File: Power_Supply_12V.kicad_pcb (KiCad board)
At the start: 2 copper layers, 16 parts, among them J1 Input, J2 Output, U1 LM7812_TO220, U2 LM7912_TO220

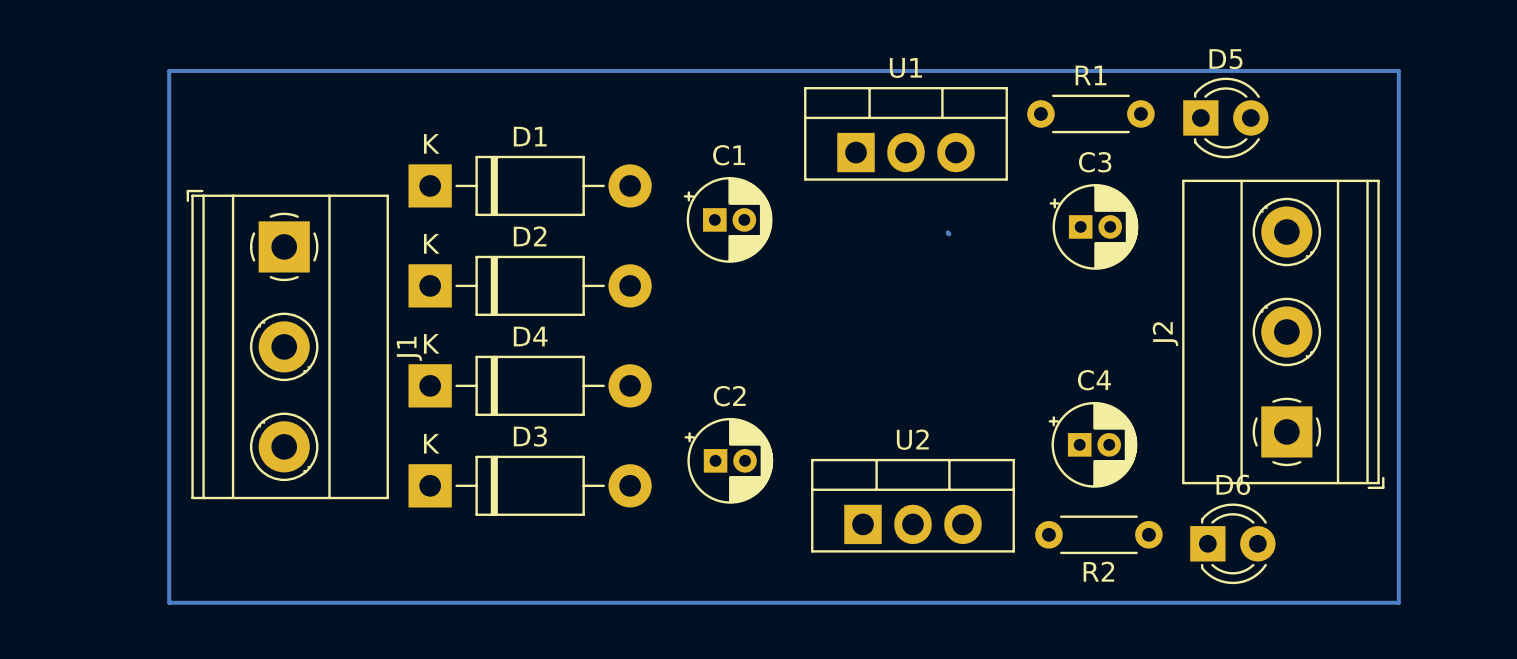
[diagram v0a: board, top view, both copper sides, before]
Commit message: Routing done
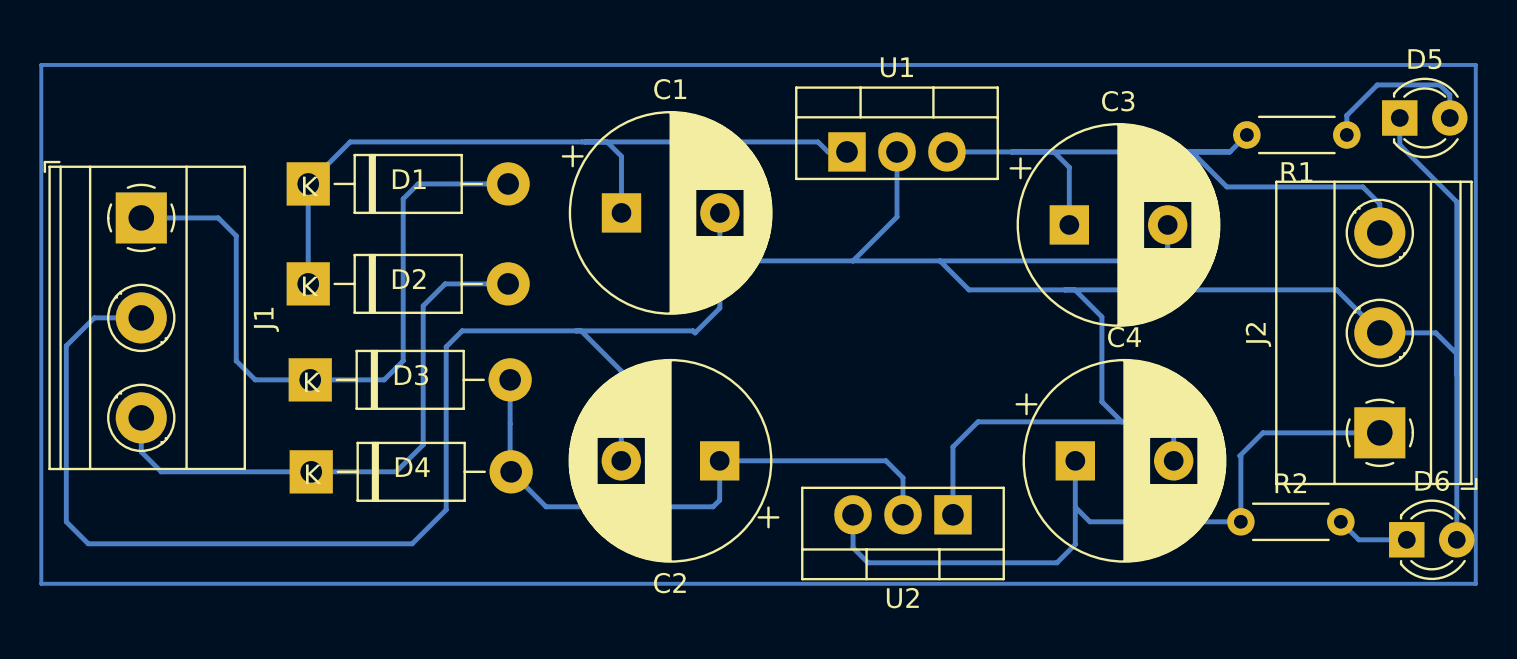
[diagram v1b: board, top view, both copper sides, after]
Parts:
- C1, C2, C3, C4: footprint Capacitor_THT:CP_Radial_D4.0mm_P1.50mm -> Capacitor_THT:CP_Radial_D10.0mm_P5.00mm
- moved R1 15.6 mm to (163.4, 68.5), turned to 180 degrees
- moved D6 10.1 mm to (166.5, 89.1)
- moved D5 10.1 mm to (166.1, 67.7)
- moved D3 8.13 mm to (110.7, 81.0)
- moved D4 7.46 mm to (110.8, 85.6)
- moved J1 7.41 mm to (102.2, 72.7)
- moved D1 6.20 mm to (110.6, 71.0)
- moved D2 6.20 mm to (110.6, 76.1)
- moved C1 4.76 mm to (126.6, 72.5)
- moved J2 4.72 mm to (165.1, 83.7)
- moved R2 4.72 mm to (158.0, 88.2), turned to 0 degrees
- moved U2 4.60 mm to (143.4, 87.8), turned to 180 degrees
- moved C4 0.84 mm to (149.6, 85.1)
- moved C3 0.59 mm to (149.3, 73.1)
- moved U1 0.46 mm to (138.0, 69.4)
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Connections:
- C3 pad 1: Net-(J2-Pin_1) -> Net-(J2-Pin_3)
- C3 pad 2: Net-(C3-Pad2) -> Net-(D5-K)
- C4 pad 1: Net-(J2-Pin_3) -> Net-(J2-Pin_1)
- C4 pad 2: Net-(C3-Pad2) -> Net-(D5-K)
- R1 pad 2: Net-(J2-Pin_1) -> Net-(J2-Pin_3)
- R2 pad 1: Net-(J2-Pin_3) -> Net-(J2-Pin_1)
- U1 pad 3: Net-(J2-Pin_1) -> Net-(J2-Pin_3)
- U2 pad 3: Net-(J2-Pin_3) -> Net-(J2-Pin_1)
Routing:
- net Net-(D5-K): track 0.61 -> 177.2 mm
- net Net-(D1-K): track 0.72 -> 38.6 mm
- net Net-(J2-Pin_1): track 0.07 -> 37.6 mm
- net Net-(J2-Pin_3): track 0.00 -> 36.9 mm
- net Net-(D1-A): track 0.00 -> 34.7 mm
- net Net-(D3-A): track 0.00 -> 30.4 mm
- net Net-(D2-A): track 0.72 -> 28.9 mm
- net Net-(D5-A): track 0.00 -> 8.24 mm
- net Net-(D6-K): track 0.00 -> 3.73 mm
